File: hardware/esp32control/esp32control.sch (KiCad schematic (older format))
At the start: 62 parts, among them J1 Conn_02x10_Odd_Even, Q5 BSS138, Q6 BSS138, Q7 MMBT3904, Q8 MMBT3904, SW1 Boot, SW2 Reset, U1 ESP32-WROOM, U10 LTV-354T, U11 HUT4, U12 LM1117-3.3, U13 RV-8523-C3, U4 LM2675M-5, U5 LTV-354T, U8 LTV-354T, U9 LTV-354T

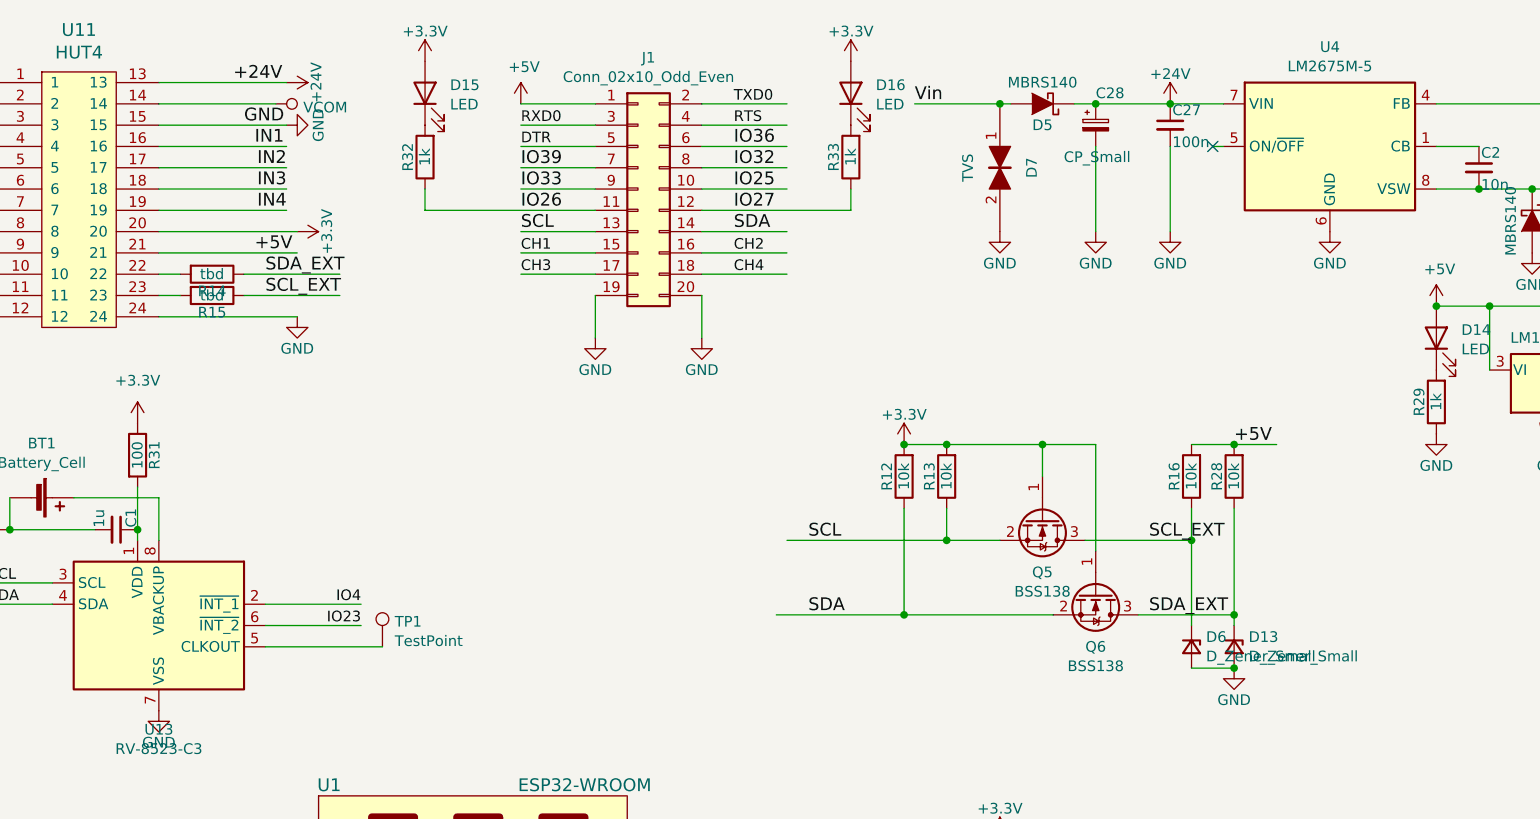
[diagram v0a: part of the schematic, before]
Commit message: bom update
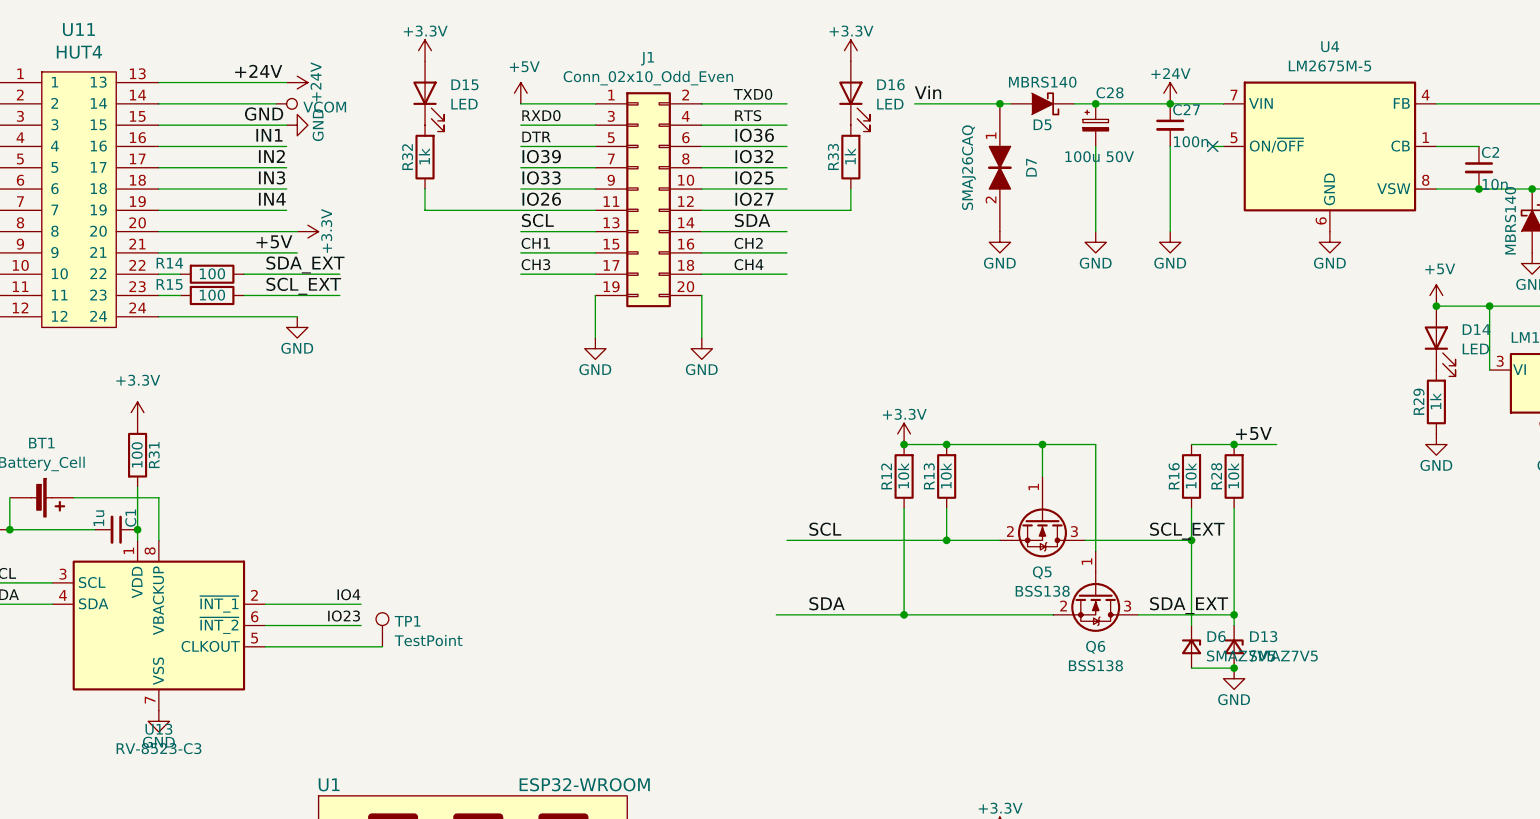
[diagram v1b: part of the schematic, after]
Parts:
- BT1: Mouser (none) -> 534-3001
- C28: value CP_Small -> 100u 50V; Mouser (none) -> 140-RGA101M1HBK0811G
- D13, D6: value D_Zener_Small -> SMAZ7V5; Mouser (none) -> 621-SMAZ7V5-F
- D4, D5: Mouser (none) -> 863-MBRS140T3G
- D7: value TVS -> SMAJ26CAQ; Mouser (none) -> 621-SMAJ26CAQ-13-F
- Q5, Q6: Mouser (none) -> 771-BSS138P215
- Q7, Q8: Mouser (none) -> 771-MMBT3904VL
- R14, R15: value tbd -> 100
- SW1, SW2: Mouser (none) -> 667-EVQ-Q2B03W
- U10, U5, U8, U9: Mouser (none) -> 859-LTV-354T
- U12: Mouser (none) -> 926-LM1117MP-3.3NOPB
- U13: Mouser (none) -> 428-201904-MG01
- U4: Mouser (none) -> 926-LM2675M-5.0/NOPB
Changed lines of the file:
@@
 F 2 "switches:SMD_Switch_6.5x6" H 7550 5900 60  0001 C CNN
 F 3 "" H 7550 5900 60  0000 C CNN
+F 4 " 667-EVQ-Q2B03W " H 7550 5900 50  0001 C CNN "Mouser"
 	1    7550 5900
 	1    0    0    -1
@@
 F 2 "Diode_SMD:D_SMA" H 10350 1550 60  0001 C CNN
 F 3 "" H 10350 1550 60  0000 C CNN
+F 4 " 863-MBRS140T3G " H 10350 1550 50  0001 C CNN "Mouser"
 	1    10350 1550
 	0    1    1    0
@@
 F 2 "Diode_SMD:D_SMA" H 8050 1000 60  0001 C CNN
 F 3 "" H 8050 1000 60  0000 C CNN
+F 4 " 863-MBRS140T3G " H 8050 1000 50  0001 C CNN "Mouser"
 	1    8050 1000
 	-1   0    0    1
@@
 P 8300 1100
 F 0 "C28" H 8300 1250 50  0000 L CNN
-F 1 "CP_Small" H 8150 950 50  0000 L CNN
+F 1 "100u 50V" H 8150 950 50  0000 L CNN
 F 2 "Capacitor_THT:CP_Radial_D8.0mm_P3.50mm" H 8300 1100 60  0001 C CNN
 F 3 "" H 8300 1100 60  0000 C CNN
+F 4 " 140-RGA101M1HBK0811G " H 8300 1100 50  0001 C CNN "Mouser"
 	1    8300 1100
 	1    0    0    -1
@@
 P 7850 1300
 F 0 "D7" H 7850 1450 50  0000 C CNN
-F 1 "TVS" H 7850 1150 50  0000 C CNN
+F 1 "SMAJ26CAQ" H 7850 1150 50  0000 C CNN
 F 2 "Diode_SMD:D_SMA" H 7850 1300 60  0001 C CNN
 F 3 "" H 7850 1300 60  0000 C CNN
+F 4 " 621-SMAJ26CAQ-13-F " H 7850 1300 50  0001 C CNN "Mouser"
 	1    7850 1300
 	0    1    1    0
@@
 F 2 "switches:SMD_Switch_6.5x6" H 7500 4850 60  0001 C CNN
 F 3 "" H 7500 4850 60  0000 C CNN
+F 4 " 667-EVQ-Q2B03W " H 7500 4850 50  0001 C CNN "Mouser"
 	1    7500 4850
 	1    0    0    -1
@@
 F 2 "SOIC_Packages:SO-4_4.4x3.6mm_Pitch2.54mm" H 1750 4750 50  0001 L CIN
 F 3 "http://optoelectronics.liteon.com/upload/download/DS70-2001-004/S_110_LTV-354T%2020140520.pdf" H 1975 4950 50  0001 L CNN
+F 4 " 859-LTV-354T " H 1950 4950 50  0001 C CNN "Mouser"
 	1    1950 4950
 	1    0    0    -1
@@
 F 2 "SOIC_Packages:SO-4_4.4x3.6mm_Pitch2.54mm" H 1750 5400 50  0001 L CIN
 F 3 "http://optoelectronics.liteon.com/upload/download/DS70-2001-004/S_110_LTV-354T%2020140520.pdf" H 1975 5600 50  0001 L CNN
+F 4 " 859-LTV-354T " H 1950 5600 50  0001 C CNN "Mouser"
 	1    1950 5600
 	1    0    0    -1
@@
 F 2 "SOIC_Packages:SO-4_4.4x3.6mm_Pitch2.54mm" H 1750 6350 50  0001 L CIN
 F 3 "http://optoelectronics.liteon.com/upload/download/DS70-2001-004/S_110_LTV-354T%2020140520.pdf" H 1975 6550 50  0001 L CNN
+F 4 " 859-LTV-354T " H 1950 6550 50  0001 C CNN "Mouser"
 	1    1950 6550
 	1    0    0    -1
@@
 F 2 "SOIC_Packages:SO-4_4.4x3.6mm_Pitch2.54mm" H 1750 7000 50  0001 L CIN
 F 3 "http://optoelectronics.liteon.com/upload/download/DS70-2001-004/S_110_LTV-354T%2020140520.pdf" H 1975 7200 50  0001 L CNN
+F 4 " 859-LTV-354T " H 1950 7200 50  0001 C CNN "Mouser"
 	1    1950 7200
 	1    0    0    -1
@@
 F 2 "Package_TO_SOT_SMD:SOT-23" H 8250 2875 50  0001 L CIN
 F 3 "https://www.fairchildsemi.com/datasheets/BS/BSS138.pdf" H 8050 2950 50  0001 L CNN
+F 4 " 771-BSS138P215 " H 8050 2950 50  0001 C CNN "Mouser"
 	1    8050 2950
 	0    1    1    0
@@
 F 2 "Package_TO_SOT_SMD:SOT-23" H 8500 3225 50  0001 L CIN
 F 3 "https://www.fairchildsemi.com/datasheets/BS/BSS138.pdf" H 8300 3300 50  0001 L CNN
+F 4 " 771-BSS138P215 " H 8300 3300 50  0001 C CNN "Mouser"
 	1    8300 3300
 	0    1    1    0
@@
 F 2 "SOIC_Packages:SOIC-8_3.9x4.9mm_Pitch1.27mm" H 9450 850 50  0001 L CIN
 F 3 "http://www.ti.com/lit/ds/symlink/lm2675.pdf" H 9400 1200 50  0001 C CNN
+F 4 " 926-LM2675M-5.0/NOPB " H 9400 1200 50  0001 C CNN "Mouser"
 	1    9400 1200
 	1    0    0    -1
@@
 F 2 "Package_TO_SOT_SMD:SOT-223-3_TabPin2" H 10450 2250 50  0001 C CNN
 F 3 "http://www.ti.com/lit/ds/symlink/lm1117.pdf" H 10450 2250 50  0001 C CNN
+F 4 " 926-LM1117MP-3.3NOPB " H 10450 2250 50  0001 C CNN "Mouser"
 	1    10450 2250
 	1    0    0    -1
@@
 U 1 1 5C2A8FC7
 P 4150 1900
-F 0 "R15" V 4230 1900 50  0000 C CNN
-F 1 "tbd" V 4150 1900 50  0000 C CNN
+F 0 "R15" V 4100 1700 50  0000 C CNN
+F 1 "100" V 4150 1900 50  0000 C CNN
 F 2 "Resistor_SMD:R_0603_1608Metric" V 4080 1900 30  0001 C CNN
 F 3 "" H 4150 1900 30  0000 C CNN
@@
 U 1 1 5C2A904F
 P 4150 1800
-F 0 "R14" V 4230 1800 50  0000 C CNN
-F 1 "tbd" V 4150 1800 50  0000 C CNN
+F 0 "R14" V 4100 1600 50  0000 C CNN
+F 1 "100" V 4150 1800 50  0000 C CNN
 F 2 "Resistor_SMD:R_0603_1608Metric" V 4080 1800 30  0001 C CNN
 F 3 "" H 4150 1800 30  0000 C CNN
@@
 P 8950 3550
 F 0 "D13" V 8904 3618 50  0000 L CNN
-F 1 "D_Zener_Small" V 8995 3618 50  0000 L CNN
+F 1 "SMAZ7V5" V 8995 3618 50  0000 L CNN
 F 2 "Diode_SMD:D_SMA" V 8950 3550 50  0001 C CNN
 F 3 "~" V 8950 3550 50  0001 C CNN
+F 4 " 621-SMAZ7V5-F " H 8950 3550 50  0001 C CNN "Mouser"
 	1    8950 3550
 	0    1    1    0
@@
 P 8750 3550
 F 0 "D6" V 8704 3618 50  0000 L CNN
-F 1 "D_Zener_Small" V 8795 3618 50  0000 L CNN
+F 1 "SMAZ7V5" V 8795 3618 50  0000 L CNN
 F 2 "Diode_SMD:D_SMA" V 8750 3550 50  0001 C CNN
 F 3 "~" V 8750 3550 50  0001 C CNN
+F 4 " 621-SMAZ7V5-F " H 8750 3550 50  0001 C CNN "Mouser"
 	1    8750 3550
 	0    1    1    0
@@
 F 2 "Package_TO_SOT_SMD:SOT-23" H 9350 5025 50  0001 L CIN
 F 3 "https://www.fairchildsemi.com/datasheets/2N/2N3904.pdf" H 9150 5100 50  0001 L CNN
+F 4 " 771-MMBT3904VL " H 9150 5100 50  0001 C CNN "Mouser"
 	1    9150 5100
 	-1   0    0    -1
@@
 F 2 "Package_TO_SOT_SMD:SOT-23" H 9350 5625 50  0001 L CIN
 F 3 "https://www.fairchildsemi.com/datasheets/2N/2N3904.pdf" H 9150 5700 50  0001 L CNN
+F 4 " 771-MMBT3904VL " H 9150 5700 50  0001 C CNN "Mouser"
 	1    9150 5700
 	-1   0    0    1
@@
 F 2 "Battery:BatteryHolder_Keystone_3001_1x12mm" V 3300 2910 50  0001 C CNN
 F 3 "~" V 3300 2910 50  0001 C CNN
+F 4 " 534-3001 " H 3300 2850 50  0001 C CNN "Mouser"
 	1    3300 2850
 	0    1    1    0
@@
 F 2 "Package_SON:RTC_SMD_MicroCrystal_C3_2.5x3.7mm" H 4900 3100 50  0001 C CNN
 F 3 "https://www.microcrystal.com/fileadmin/Media/Products/RTC/Datasheet/RV-8523-C3.pdf" H 3900 3450 50  0001 C CNN
+F 4 " 428-201904-MG01 " H 3900 3450 50  0001 C CNN "Mouser"
 	1    3900 3450
 	1    0    0    -1
